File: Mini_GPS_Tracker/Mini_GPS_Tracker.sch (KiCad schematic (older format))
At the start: 17 parts, among them J1 USB_C_Receptacle, J4 Conn_ARM_JTAG_SWD_10, SW1 SW_Push, U11 STM32F413ZHTx, Y1 32.786 KHz

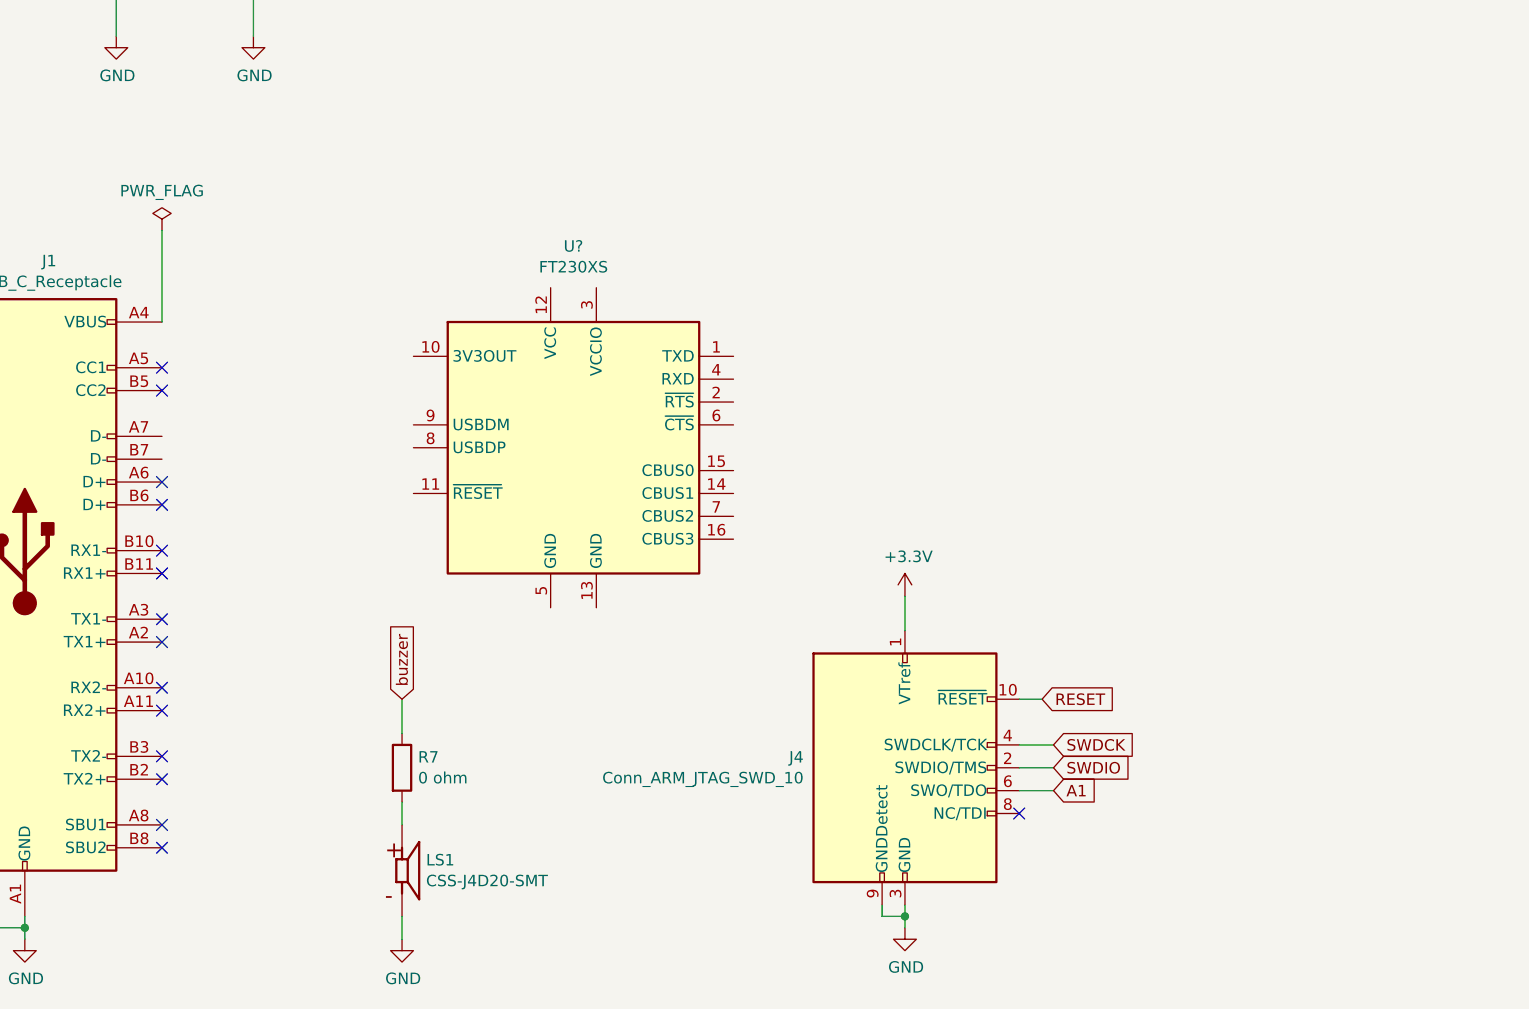
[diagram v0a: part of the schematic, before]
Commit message: added back usb circuit
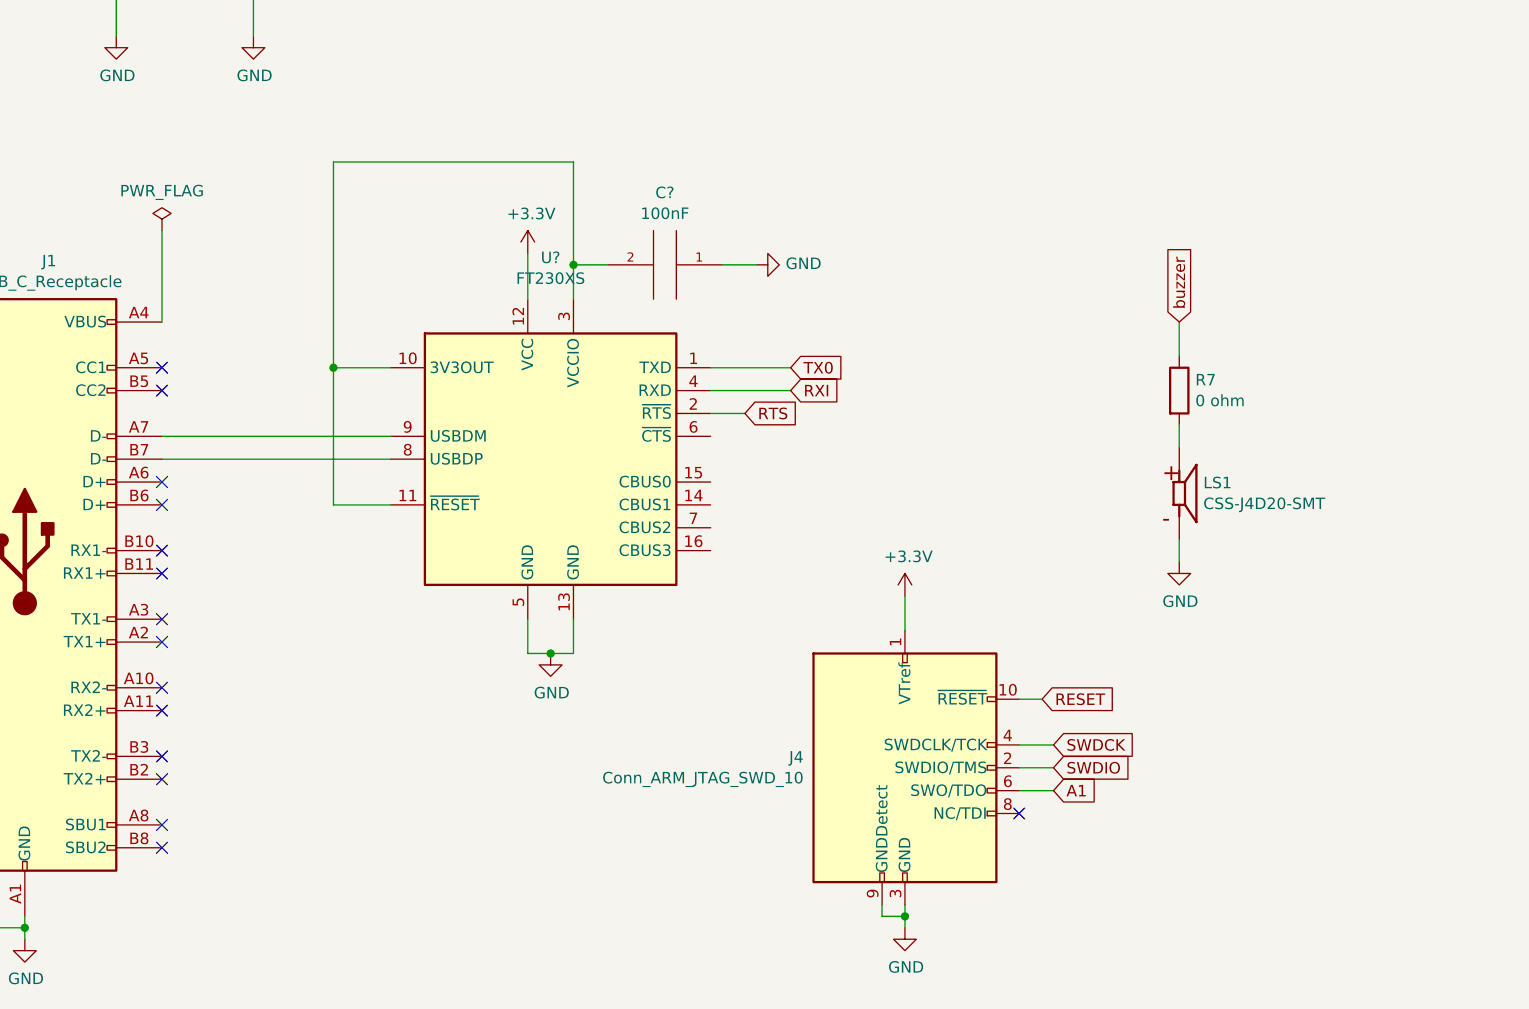
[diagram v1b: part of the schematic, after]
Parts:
- added C?: 100nF, symbol pspice:CAP
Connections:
- wire segments 72 -> 91
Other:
- moved on the sheet: LS1, R7, U?
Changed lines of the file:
@@
 L Mini_GPS_Tracker-rescue:CSS-J4D20-SMT-Sparkfun_Artemis-Mini_GPS_Tracker-rescue LS1
 U 1 1 5E7E01A2
-P 2850 7050
-F 0 "LS1" H 2955 7096 50  0000 L CNN
-F 1 "CSS-J4D20-SMT" H 2955 7005 50  0000 L CNN
-F 2 "Sparkfun-Artemis:CUI_CSS-J4D20-SMT" H 2850 7050 50  0001 L BNN
-F 3 "CUI" H 2850 7050 50  0001 L BNN
-F 4 "None" H 2850 7050 50  0001 L BNN "Field4"
-F 5 "CSS-J4D20-SMT" H 2850 7050 50  0001 L BNN "Field5"
-F 6 "Unavailable" H 2850 7050 50  0001 L BNN "Field6"
-F 7 "8.5 mm, 3.6 V, 90 dB, Surface Mount _SMT_, Magnetic Audio Transducer Buzzer" H 2850 7050 50  0001 L BNN "Field7"
-F 8 "None" H 2850 7050 50  0001 L BNN "Field8"
-	1    2850 7050
+P 6250 5400
+F 0 "LS1" H 6355 5446 50  0000 L CNN
+F 1 "CSS-J4D20-SMT" H 6355 5355 50  0000 L CNN
+F 2 "Sparkfun-Artemis:CUI_CSS-J4D20-SMT" H 6250 5400 50  0001 L BNN
+F 3 "CUI" H 6250 5400 50  0001 L BNN
+F 4 "None" H 6250 5400 50  0001 L BNN "Field4"
+F 5 "CSS-J4D20-SMT" H 6250 5400 50  0001 L BNN "Field5"
+F 6 "Unavailable" H 6250 5400 50  0001 L BNN "Field6"
+F 7 "8.5 mm, 3.6 V, 90 dB, Surface Mount _SMT_, Magnetic Audio Transducer Buzzer" H 6250 5400 50  0001 L BNN "Field7"
+F 8 "None" H 6250 5400 50  0001 L BNN "Field8"
+	1    6250 5400
 	1    0    0    -1
 $EndComp
@@
 L Device:R R7
 U 1 1 5E7E2738
-P 2850 6600
-F 0 "R7" H 2920 6646 50  0000 L CNN
-F 1 "0 ohm" H 2920 6555 50  0000 L CNN
-F 2 "Resistor_SMD:R_0805_2012Metric_Pad1.15x1.40mm_HandSolder" V 2780 6600 50  0001 C CNN
-F 3 "~" H 2850 6600 50  0001 C CNN
-	1    2850 6600
+P 6250 4950
+F 0 "R7" H 6320 4996 50  0000 L CNN
+F 1 "0 ohm" H 6320 4905 50  0000 L CNN
+F 2 "Resistor_SMD:R_0805_2012Metric_Pad1.15x1.40mm_HandSolder" V 6180 4950 50  0001 C CNN
+F 3 "~" H 6250 4950 50  0001 C CNN
+	1    6250 4950
 	1    0    0    -1
 $EndComp
@@
 L power:GND #PWR0116
 U 1 1 5E7E36E3
-P 2850 7350
-F 0 "#PWR0116" H 2850 7100 50  0001 C CNN
-F 1 "GND" H 2855 7177 50  0000 C CNN
-F 2 "" H 2850 7350 50  0001 C CNN
-F 3 "" H 2850 7350 50  0001 C CNN
-	1    2850 7350
-	1    0    0    -1
-$EndComp
-Wire Wire Line
-	2850 7250 2850 7350
-Wire Wire Line
-	2850 6850 2850 6750
-Text GLabel 2850 6300 1    50   Input ~ 0
+P 6250 5700
+F 0 "#PWR0116" H 6250 5450 50  0001 C CNN
+F 1 "GND" H 6255 5527 50  0000 C CNN
+F 2 "" H 6250 5700 50  0001 C CNN
+F 3 "" H 6250 5700 50  0001 C CNN
+	1    6250 5700
+	1    0    0    -1
+$EndComp
+Wire Wire Line
+	6250 5600 6250 5700
+Wire Wire Line
+	6250 5200 6250 5100
+Text GLabel 6250 4650 1    50   Input ~ 0
 buzzer
 Wire Wire Line
-	2850 6300 2850 6450
+	6250 4650 6250 4800
 Text GLabel 8250 3950 2    50   Input ~ 0
 buzzer
@@
 L Interface_USB:FT230XS U?
 U 1 1 5E9B8EAD
-P 3600 5200
-F 0 "U?" H 3600 6081 50  0000 C CNN
-F 1 "FT230XS" H 3600 5990 50  0000 C CNN
-F 2 "Package_SO:SSOP-16_3.9x4.9mm_P0.635mm" H 4600 4600 50  0001 C CNN
-F 3 "https://www.ftdichip.com/Support/Documents/DataSheets/ICs/DS_FT230X.pdf" H 3600 5200 50  0001 C CNN
-	1    3600 5200
-	1    0    0    -1
-$EndComp
+P 3500 5250
+F 0 "U?" H 3500 6131 50  0000 C CNN
+F 1 "FT230XS" H 3500 6040 50  0000 C CNN
+F 2 "Package_SO:SSOP-16_3.9x4.9mm_P0.635mm" H 4500 4650 50  0001 C CNN
+F 3 "https://www.ftdichip.com/Support/Documents/DataSheets/ICs/DS_FT230X.pdf" H 3500 5250 50  0001 C CNN
+	1    3500 5250
+	1    0    0    -1
+$EndComp
+Wire Wire Line
+	1800 5150 2800 5150
+Wire Wire Line
+	1800 5250 2800 5250
+$Comp
+L power:GND #PWR?
+U 1 1 5E9DAEFA
+P 3500 6100
+F 0 "#PWR?" H 3500 5850 50  0001 C CNN
+F 1 "GND" H 3505 5927 50  0000 C CNN
+F 2 "" H 3500 6100 50  0001 C CNN
+F 3 "" H 3500 6100 50  0001 C CNN
+	1    3500 6100
+	1    0    0    -1
+$EndComp
+Wire Wire Line
+	3400 5950 3400 6100
+Wire Wire Line
+	3400 6100 3500 6100
+Wire Wire Line
+	3500 6100 3600 6100
+Wire Wire Line
+	3600 6100 3600 5950
+Connection ~ 3500 6100
+Text GLabel 4350 5050 2    50   Input ~ 0
+RTS
+Wire Wire Line
+	4200 5050 4350 5050
+Text GLabel 4550 4950 2    50   Input ~ 0
+RXI
+Text GLabel 4550 4850 2    50   Input ~ 0
+TX0
+Wire Wire Line
+	4200 4850 4550 4850
+Wire Wire Line
+	4200 4950 4550 4950
+$Comp
+L power:+3.3V #PWR?
+U 1 1 5E9E8361
+P 3400 4350
+F 0 "#PWR?" H 3400 4200 50  0001 C CNN
+F 1 "+3.3V" H 3415 4523 50  0000 C CNN
+F 2 "" H 3400 4350 50  0001 C CNN
+F 3 "" H 3400 4350 50  0001 C CNN
+	1    3400 4350
+	1    0    0    -1
+$EndComp
+Wire Wire Line
+	3400 4550 3400 4350
+$Comp
+L pspice:CAP C?
+U 1 1 5E9EBAC9
+P 4000 4400
+F 0 "C?" V 3685 4400 50  0000 C CNN
+F 1 "100nF" V 3776 4400 50  0000 C CNN
+F 2 "" H 4000 4400 50  0001 C CNN
+F 3 "~" H 4000 4400 50  0001 C CNN
+	1    4000 4400
+	0    1    1    0
+$EndComp
+$Comp
+L power:GND #PWR?
+U 1 1 5E9EC72D
+P 4400 4400
+F 0 "#PWR?" H 4400 4150 50  0001 C CNN
+F 1 "GND" V 4405 4272 50  0000 R CNN
+F 2 "" H 4400 4400 50  0001 C CNN
+F 3 "" H 4400 4400 50  0001 C CNN
+	1    4400 4400
+	0    -1   -1   0
+$EndComp
+Wire Wire Line
+	4250 4400 4400 4400
+Wire Wire Line
+	2800 5450 2550 5450
+Wire Wire Line
+	2550 5450 2550 4850
+Wire Wire Line
+	2550 3950 3600 3950
+Wire Wire Line
+	3600 3950 3600 4400
+Wire Wire Line
+	3750 4400 3600 4400
+Connection ~ 3600 4400
+Wire Wire Line
+	3600 4400 3600 4550
+Wire Wire Line
+	2800 4850 2550 4850
+Connection ~ 2550 4850
+Wire Wire Line
+	2550 4850 2550 3950
 $EndSCHEMATC
